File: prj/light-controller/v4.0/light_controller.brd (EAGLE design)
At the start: 195.6 x 254.5 mm, 239 parts, among them J2 PJ-036AH, J4 54602-908LF, J8 54602-908LF, Q1 MMBT2222A, Q2 MMBT2222A, Q3 MMBT2222A, Q4 MMBT2222A, Q5 MMBT2222A, Q6 MMBT2222A, Q7 MMBT2222A, Q8 MMBT2222A, U11 PCA9615, U13 LM2937-3.3V, U17 R-78E5.0-1.0, U7 DAC5578

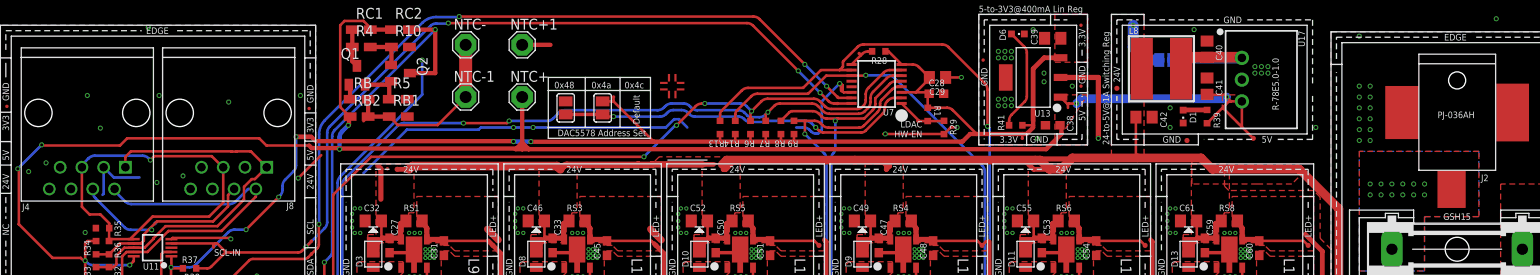
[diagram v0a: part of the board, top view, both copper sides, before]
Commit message: Added boards (Relay, Display, GPIO, etc)
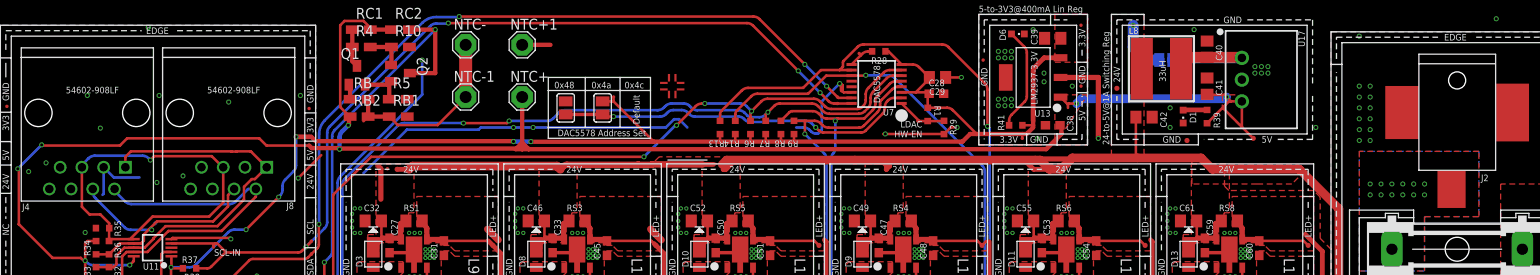
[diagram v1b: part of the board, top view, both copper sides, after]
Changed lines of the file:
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@@
 <attribute name="MPN" value="29333C" x="97.282" y="60.96" size="0.762" layer="27" display="off"/>
 <attribute name="NAME" x="93.472" y="65.024" size="0.762" layer="25"/>
+<attribute name="VALUE" x="97.79" y="59.436" size="0.762" layer="27" rot="R90"/>
 <attribute name="VALUE" x="97.79" y="59.436" size="0.762" layer="21" rot="R90"/>
-<attribute name="VALUE" x="97.79" y="59.436" size="0.762" layer="27" rot="R90"/>
 <attribute name="VENDOR" value="Digikey" x="97.282" y="60.96" size="0.762" layer="27" display="off"/>
 <attribute name="VLINK" value="https://www.digikey.com/product-detail/en/murata-power-solutions-inc/29333C/811-1138-1-ND/1924860" x="97.282" y="60.96" size="0.762" layer="27" display="off"/>
@@
 <attribute name="MPN" value="R-78E5.0-1.0" x="106.68" y="59.69" size="0.762" layer="27" rot="R270" display="off"/>
 <attribute name="NAME" x="113.284" y="65.405" size="0.762" layer="25" rot="R270"/>
+<attribute name="VALUE" x="110.236" y="62.23" size="0.762" layer="21" rot="R270"/>
 <attribute name="VALUE" x="110.236" y="62.23" size="0.762" layer="27" rot="R270"/>
-<attribute name="VALUE" x="110.236" y="62.23" size="0.762" layer="21" rot="R270"/>
 <attribute name="VENDOR" value="Digikey" x="106.68" y="59.69" size="0.762" layer="27" rot="R270" display="off"/>
 <attribute name="VLINK" value="https://www.digikey.com/product-detail/en/recom-power/R-78E5.0-1.0/945-2201-ND/4930585" x="106.68" y="59.69" size="0.762" layer="27" rot="R270" display="off"/>
@@
 <attribute name="MPN" value="54602-908LF" x="-28.194" y="55.8038" size="0.762" layer="27" rot="R180" display="off"/>
 <attribute name="NAME" x="-35.814" y="44.4373" size="0.762" layer="25"/>
+<attribute name="VALUE" x="-24.511" y="58.8518" size="0.762" layer="27" rot="R180"/>
 <attribute name="VALUE" x="-24.511" y="58.8518" size="0.762" layer="21" rot="R180"/>
-<attribute name="VALUE" x="-24.511" y="58.8518" size="0.762" layer="27" rot="R180"/>
 <attribute name="VENDOR" value="Digikey" x="-28.194" y="55.8038" size="0.762" layer="27" rot="R180" display="off"/>
 <attribute name="VLINK" value="https://www.digikey.com/product-detail/en/amphenol-fci/54602-908LF/609-1046-ND/1001360" x="-28.194" y="55.8038" size="0.762" layer="27" rot="R180" display="off"/>
@@
 <attribute name="MPN" value="54602-908LF" x="-11.684" y="55.8038" size="0.762" layer="27" rot="R180" display="off"/>
 <attribute name="NAME" x="-4.064" y="45.3263" size="0.762" layer="25" rot="R180"/>
+<attribute name="VALUE" x="-8.001" y="58.8518" size="0.762" layer="27" rot="R180"/>
 <attribute name="VALUE" x="-8.001" y="58.8518" size="0.762" layer="21" rot="R180"/>
-<attribute name="VALUE" x="-8.001" y="58.8518" size="0.762" layer="27" rot="R180"/>
 <attribute name="VENDOR" value="Digikey" x="-11.684" y="55.8038" size="0.762" layer="27" rot="R180" display="off"/>
 <attribute name="VLINK" value="https://www.digikey.com/product-detail/en/amphenol-fci/54602-908LF/609-1046-ND/1001360" x="-11.684" y="55.8038" size="0.762" layer="27" rot="R180" display="off"/>
@@
 <attribute name="MPN" value="PJ-036AH-SMT-TR" x="131.826" y="49.0982" size="1.778" layer="27" rot="R270" display="off"/>
 <attribute name="NAME" x="134.62" y="47.8282" size="0.762" layer="21"/>
+<attribute name="VALUE" x="129.54" y="55.1942" size="0.762" layer="21"/>
 <attribute name="VALUE" x="129.54" y="55.1942" size="0.762" layer="27"/>
-<attribute name="VALUE" x="129.54" y="55.1942" size="0.762" layer="21"/>
 <attribute name="VENDOR" value="Digikey" x="131.826" y="49.0982" size="1.778" layer="27" rot="R270" display="off"/>
 <attribute name="VLINK" value="https://www.digikey.com/product-detail/en/cui-inc/PJ-036AH-SMT-TR/CP-036AHPJCT-ND/1530994" x="131.826" y="49.0982" size="1.778" layer="27" rot="R270" display="off"/>
@@
 <attribute name="MPN" value="DAC5578SPW" x="64.008" y="59.182" size="1.778" layer="27" rot="R90" display="off"/>
 <attribute name="NAME" x="66.04" y="56.261" size="0.762" layer="25" rot="R180"/>
+<attribute name="VALUE" x="64.423" y="56.948" size="0.762" layer="27" rot="R90"/>
 <attribute name="VALUE" x="64.423" y="56.948" size="0.762" layer="21" rot="R90"/>
-<attribute name="VALUE" x="64.423" y="56.948" size="0.762" layer="27" rot="R90"/>
 <attribute name="VENDOR" value="Digikey" x="64.008" y="59.182" size="1.778" layer="27" rot="R90" display="off"/>
 <attribute name="VLINK" value="https://www.digikey.com/product-detail/en/texas-instruments/DAC5578SPW/296-27736-5-ND/2360827" x="64.008" y="59.182" size="1.778" layer="27" rot="R90" display="off"/>
@@
 <attribute name="MPN" value="LM2937IMP-3.3/NOPB" x="82.296" y="59.944" size="1.778" layer="27" rot="R180" display="off"/>
 <attribute name="NAME" x="84.328" y="56.134" size="0.762" layer="25" ratio="6" rot="R180"/>
+<attribute name="VALUE" x="82.042" y="62.992" size="0.762" layer="27" ratio="6" rot="R270"/>
 <attribute name="VALUE" x="82.042" y="62.992" size="0.762" layer="21" ratio="6" rot="R270"/>
-<attribute name="VALUE" x="82.042" y="62.992" size="0.762" layer="27" ratio="6" rot="R270"/>
 <attribute name="VENDOR" value="Digikey" x="82.296" y="59.944" size="1.778" layer="27" rot="R180" display="off"/>
 <attribute name="VLINK" value="https://www.digikey.com/product-detail/en/texas-instruments/LM2937IMP-3.3-NOPB/LM2937IMP-3.3-NOPBCT-ND/270742#" x="82.296" y="59.944" size="1.778" layer="27" rot="R180" display="off"/>
@@
 <attribute name="MPN" value="64900001039" x="131.826" y="39.878" size="0.762" layer="27" display="off"/>
 <attribute name="NAME" x="119.2784" y="34.0868" size="0.762" layer="25" ratio="10"/>
+<attribute name="VALUE" x="130.2004" y="43.307" size="0.762" layer="21" ratio="10"/>
 <attribute name="VALUE" x="130.2004" y="43.307" size="0.762" layer="27" ratio="10"/>
-<attribute name="VALUE" x="130.2004" y="43.307" size="0.762" layer="21" ratio="10"/>
 <attribute name="VENDOR" value="Digikey" x="131.826" y="39.878" size="0.762" layer="27" display="off"/>
 <attribute name="VLINK" value="https://www.digikey.com/product-detail/en/littelfuse-inc/64900001039/WK0011-ND/245470" x="131.826" y="39.878" size="0.762" layer="27" display="off"/>

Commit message: added fermentaboard, etc
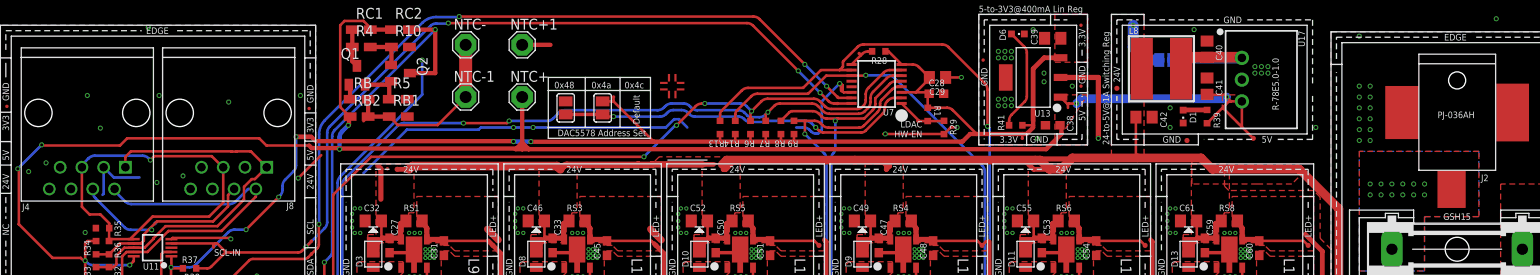
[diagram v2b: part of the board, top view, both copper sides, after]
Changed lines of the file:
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@@
 <attribute name="MPN" value="29333C" x="97.282" y="60.96" size="0.762" layer="27" display="off"/>
 <attribute name="NAME" x="93.472" y="65.024" size="0.762" layer="25"/>
+<attribute name="VALUE" x="97.79" y="59.436" size="0.762" layer="21" rot="R90"/>
 <attribute name="VALUE" x="97.79" y="59.436" size="0.762" layer="27" rot="R90"/>
-<attribute name="VALUE" x="97.79" y="59.436" size="0.762" layer="21" rot="R90"/>
 <attribute name="VENDOR" value="Digikey" x="97.282" y="60.96" size="0.762" layer="27" display="off"/>
 <attribute name="VLINK" value="https://www.digikey.com/product-detail/en/murata-power-solutions-inc/29333C/811-1138-1-ND/1924860" x="97.282" y="60.96" size="0.762" layer="27" display="off"/>
@@
 <attribute name="MPN" value="R-78E5.0-1.0" x="106.68" y="59.69" size="0.762" layer="27" rot="R270" display="off"/>
 <attribute name="NAME" x="113.284" y="65.405" size="0.762" layer="25" rot="R270"/>
+<attribute name="VALUE" x="110.236" y="62.23" size="0.762" layer="27" rot="R270"/>
 <attribute name="VALUE" x="110.236" y="62.23" size="0.762" layer="21" rot="R270"/>
-<attribute name="VALUE" x="110.236" y="62.23" size="0.762" layer="27" rot="R270"/>
 <attribute name="VENDOR" value="Digikey" x="106.68" y="59.69" size="0.762" layer="27" rot="R270" display="off"/>
 <attribute name="VLINK" value="https://www.digikey.com/product-detail/en/recom-power/R-78E5.0-1.0/945-2201-ND/4930585" x="106.68" y="59.69" size="0.762" layer="27" rot="R270" display="off"/>
@@
 <attribute name="MPN" value="54602-908LF" x="-28.194" y="55.8038" size="0.762" layer="27" rot="R180" display="off"/>
 <attribute name="NAME" x="-35.814" y="44.4373" size="0.762" layer="25"/>
+<attribute name="VALUE" x="-24.511" y="58.8518" size="0.762" layer="21" rot="R180"/>
 <attribute name="VALUE" x="-24.511" y="58.8518" size="0.762" layer="27" rot="R180"/>
-<attribute name="VALUE" x="-24.511" y="58.8518" size="0.762" layer="21" rot="R180"/>
 <attribute name="VENDOR" value="Digikey" x="-28.194" y="55.8038" size="0.762" layer="27" rot="R180" display="off"/>
 <attribute name="VLINK" value="https://www.digikey.com/product-detail/en/amphenol-fci/54602-908LF/609-1046-ND/1001360" x="-28.194" y="55.8038" size="0.762" layer="27" rot="R180" display="off"/>
@@
 <attribute name="MPN" value="54602-908LF" x="-11.684" y="55.8038" size="0.762" layer="27" rot="R180" display="off"/>
 <attribute name="NAME" x="-4.064" y="45.3263" size="0.762" layer="25" rot="R180"/>
+<attribute name="VALUE" x="-8.001" y="58.8518" size="0.762" layer="21" rot="R180"/>
 <attribute name="VALUE" x="-8.001" y="58.8518" size="0.762" layer="27" rot="R180"/>
-<attribute name="VALUE" x="-8.001" y="58.8518" size="0.762" layer="21" rot="R180"/>
 <attribute name="VENDOR" value="Digikey" x="-11.684" y="55.8038" size="0.762" layer="27" rot="R180" display="off"/>
 <attribute name="VLINK" value="https://www.digikey.com/product-detail/en/amphenol-fci/54602-908LF/609-1046-ND/1001360" x="-11.684" y="55.8038" size="0.762" layer="27" rot="R180" display="off"/>
@@
 <attribute name="MPN" value="PJ-036AH-SMT-TR" x="131.826" y="49.0982" size="1.778" layer="27" rot="R270" display="off"/>
 <attribute name="NAME" x="134.62" y="47.8282" size="0.762" layer="21"/>
+<attribute name="VALUE" x="129.54" y="55.1942" size="0.762" layer="27"/>
 <attribute name="VALUE" x="129.54" y="55.1942" size="0.762" layer="21"/>
-<attribute name="VALUE" x="129.54" y="55.1942" size="0.762" layer="27"/>
 <attribute name="VENDOR" value="Digikey" x="131.826" y="49.0982" size="1.778" layer="27" rot="R270" display="off"/>
 <attribute name="VLINK" value="https://www.digikey.com/product-detail/en/cui-inc/PJ-036AH-SMT-TR/CP-036AHPJCT-ND/1530994" x="131.826" y="49.0982" size="1.778" layer="27" rot="R270" display="off"/>
@@
 <attribute name="MPN" value="DAC5578SPW" x="64.008" y="59.182" size="1.778" layer="27" rot="R90" display="off"/>
 <attribute name="NAME" x="66.04" y="56.261" size="0.762" layer="25" rot="R180"/>
+<attribute name="VALUE" x="64.423" y="56.948" size="0.762" layer="21" rot="R90"/>
 <attribute name="VALUE" x="64.423" y="56.948" size="0.762" layer="27" rot="R90"/>
-<attribute name="VALUE" x="64.423" y="56.948" size="0.762" layer="21" rot="R90"/>
 <attribute name="VENDOR" value="Digikey" x="64.008" y="59.182" size="1.778" layer="27" rot="R90" display="off"/>
 <attribute name="VLINK" value="https://www.digikey.com/product-detail/en/texas-instruments/DAC5578SPW/296-27736-5-ND/2360827" x="64.008" y="59.182" size="1.778" layer="27" rot="R90" display="off"/>
@@
 <attribute name="MPN" value="LM2937IMP-3.3/NOPB" x="82.296" y="59.944" size="1.778" layer="27" rot="R180" display="off"/>
 <attribute name="NAME" x="84.328" y="56.134" size="0.762" layer="25" ratio="6" rot="R180"/>
+<attribute name="VALUE" x="82.042" y="62.992" size="0.762" layer="21" ratio="6" rot="R270"/>
 <attribute name="VALUE" x="82.042" y="62.992" size="0.762" layer="27" ratio="6" rot="R270"/>
-<attribute name="VALUE" x="82.042" y="62.992" size="0.762" layer="21" ratio="6" rot="R270"/>
 <attribute name="VENDOR" value="Digikey" x="82.296" y="59.944" size="1.778" layer="27" rot="R180" display="off"/>
 <attribute name="VLINK" value="https://www.digikey.com/product-detail/en/texas-instruments/LM2937IMP-3.3-NOPB/LM2937IMP-3.3-NOPBCT-ND/270742#" x="82.296" y="59.944" size="1.778" layer="27" rot="R180" display="off"/>
@@
 <attribute name="MPN" value="64900001039" x="131.826" y="39.878" size="0.762" layer="27" display="off"/>
 <attribute name="NAME" x="119.2784" y="34.0868" size="0.762" layer="25" ratio="10"/>
+<attribute name="VALUE" x="130.2004" y="43.307" size="0.762" layer="27" ratio="10"/>
 <attribute name="VALUE" x="130.2004" y="43.307" size="0.762" layer="21" ratio="10"/>
-<attribute name="VALUE" x="130.2004" y="43.307" size="0.762" layer="27" ratio="10"/>
 <attribute name="VENDOR" value="Digikey" x="131.826" y="39.878" size="0.762" layer="27" display="off"/>
 <attribute name="VLINK" value="https://www.digikey.com/product-detail/en/littelfuse-inc/64900001039/WK0011-ND/245470" x="131.826" y="39.878" size="0.762" layer="27" display="off"/>
